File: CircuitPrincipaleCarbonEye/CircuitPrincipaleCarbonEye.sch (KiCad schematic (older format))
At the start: 28 parts, among them J1 Conn_01x01_Male, J2 4P4C, Q1 Q_PMOS_DGS, Q2 Q_NMOS_DGS, U1 OPA4227PA, U2 ADS1115, U3 GROOVE, U4 molex4-pin

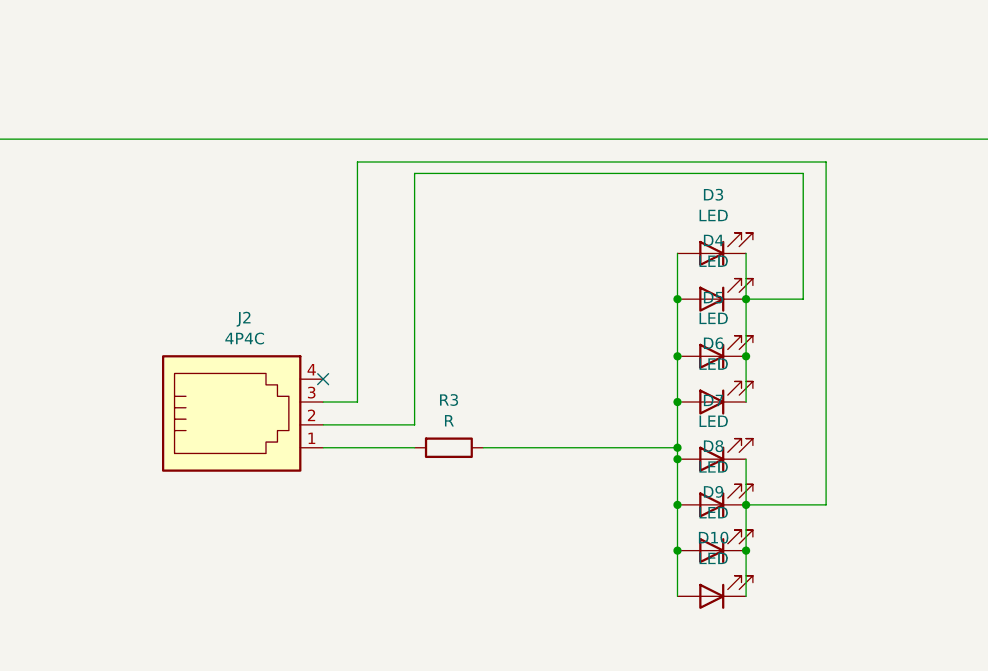
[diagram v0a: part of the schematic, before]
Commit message: CircuitLed V1.0
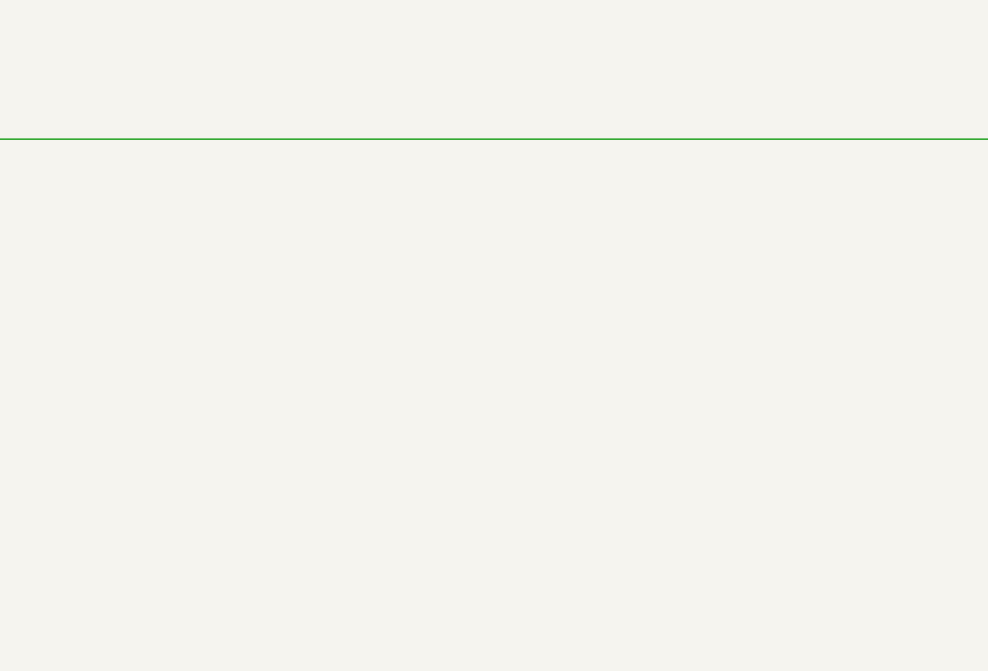
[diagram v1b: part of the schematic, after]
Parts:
- removed D10, D7, D8, D9: LED, symbol Device:LED
- removed D3, D4, D5, D6: LED, SamacSys_Parts:LEDM3528X185N, symbol Device:LED
- removed J2: 4P4C, symbol Connector:4P4C
- removed R3: R, symbol Device:R
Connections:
- no-connect marks 11 -> 10
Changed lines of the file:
@@
 Wire Wire Line
 	2150 5250 2450 5250
-$Comp
-L Connector:4P4C J2
-U 1 1 60EA57EE
-P 5950 4600
-F 0 "J2" H 6007 5067 50  0000 C CNN
-F 1 "4P4C" H 6007 4976 50  0000 C CNN
-F 2 "" V 5950 4650 50  0001 C CNN
-F 3 "~" V 5950 4650 50  0001 C CNN
-	1    5950 4600
-	1    0    0    -1
-$EndComp
-$Comp
-L Device:R R3
-U 1 1 60EA62A5
-P 6900 4700
-F 0 "R3" V 6693 4700 50  0000 C CNN
-F 1 "R" V 6784 4700 50  0000 C CNN
-F 2 "" V 6830 4700 50  0001 C CNN
-F 3 "~" H 6900 4700 50  0001 C CNN
-	1    6900 4700
-	0    1    1    0
-$EndComp
-$Comp
-L Device:LED D5
-U 1 1 60EA71C0
-P 8050 4300
-F 0 "D5" H 8043 4045 50  0000 C CNN
-F 1 "LED" H 8043 4136 50  0000 C CNN
-F 2 "SamacSys_Parts:LEDM3528X185N" H 8050 4300 50  0001 C CNN
-F 3 "~" H 8050 4300 50  0001 C CNN
-	1    8050 4300
-	-1   0    0    1
-$EndComp
-$Comp
-L Device:LED D4
-U 1 1 60EA7A9B
-P 8050 4050
-F 0 "D4" H 8043 3795 50  0000 C CNN
-F 1 "LED" H 8043 3886 50  0000 C CNN
-F 2 "SamacSys_Parts:LEDM3528X185N" H 8050 4050 50  0001 C CNN
-F 3 "~" H 8050 4050 50  0001 C CNN
-	1    8050 4050
-	-1   0    0    1
-$EndComp
-$Comp
-L Device:LED D3
-U 1 1 60EA7F32
-P 8050 3850
-F 0 "D3" H 8043 3595 50  0000 C CNN
-F 1 "LED" H 8043 3686 50  0000 C CNN
-F 2 "SamacSys_Parts:LEDM3528X185N" H 8050 3850 50  0001 C CNN
-F 3 "~" H 8050 3850 50  0001 C CNN
-	1    8050 3850
-	-1   0    0    1
-$EndComp
-$Comp
-L Device:LED D6
-U 1 1 60EA8289
-P 8050 4500
-F 0 "D6" H 8043 4245 50  0000 C CNN
-F 1 "LED" H 8043 4336 50  0000 C CNN
-F 2 "SamacSys_Parts:LEDM3528X185N" H 8050 4500 50  0001 C CNN
-F 3 "~" H 8050 4500 50  0001 C CNN
-	1    8050 4500
-	-1   0    0    1
-$EndComp
-Wire Wire Line
-	6350 4700 6750 4700
-Wire Wire Line
-	7900 3850 7900 4050
-Connection ~ 7900 4050
-Wire Wire Line
-	7900 4050 7900 4300
-Connection ~ 7900 4300
-Wire Wire Line
-	7900 4300 7900 4500
-Wire Wire Line
-	8200 3850 8200 4050
-Connection ~ 8200 4050
-Wire Wire Line
-	8200 4050 8200 4300
-Connection ~ 8200 4300
-Wire Wire Line
-	8200 4300 8200 4500
-$Comp
-L Device:LED D7
-U 1 1 60EB0F00
-P 8050 4750
-F 0 "D7" H 8043 4495 50  0000 C CNN
-F 1 "LED" H 8043 4586 50  0000 C CNN
-F 2 "" H 8050 4750 50  0001 C CNN
-F 3 "~" H 8050 4750 50  0001 C CNN
-	1    8050 4750
-	-1   0    0    1
-$EndComp
-$Comp
-L Device:LED D8
-U 1 1 60EB123F
-P 8050 4950
-F 0 "D8" H 8043 4695 50  0000 C CNN
-F 1 "LED" H 8043 4786 50  0000 C CNN
-F 2 "" H 8050 4950 50  0001 C CNN
-F 3 "~" H 8050 4950 50  0001 C CNN
-	1    8050 4950
-	-1   0    0    1
-$EndComp
-$Comp
-L Device:LED D9
-U 1 1 60EB143A
-P 8050 5150
-F 0 "D9" H 8043 4895 50  0000 C CNN
-F 1 "LED" H 8043 4986 50  0000 C CNN
-F 2 "" H 8050 5150 50  0001 C CNN
-F 3 "~" H 8050 5150 50  0001 C CNN
-	1    8050 5150
-	-1   0    0    1
-$EndComp
-$Comp
-L Device:LED D10
-U 1 1 60EB16ED
-P 8050 5350
-F 0 "D10" H 8043 5095 50  0000 C CNN
-F 1 "LED" H 8043 5186 50  0000 C CNN
-F 2 "" H 8050 5350 50  0001 C CNN
-F 3 "~" H 8050 5350 50  0001 C CNN
-	1    8050 5350
-	-1   0    0    1
-$EndComp
-Wire Wire Line
-	7900 4750 7900 4950
-Connection ~ 7900 4950
-Wire Wire Line
-	7900 4950 7900 5150
-Connection ~ 7900 5150
-Wire Wire Line
-	7900 5150 7900 5350
-Wire Wire Line
-	8200 4750 8200 4950
-Connection ~ 8200 4950
-Wire Wire Line
-	8200 4950 8200 5150
-Connection ~ 8200 5150
-Wire Wire Line
-	8200 5150 8200 5350
-Wire Wire Line
-	7050 4700 7900 4700
-Wire Wire Line
-	7900 4700 7900 4750
-Connection ~ 7900 4750
-Wire Wire Line
-	7900 4700 7900 4500
-Connection ~ 7900 4700
-Connection ~ 7900 4500
-Wire Wire Line
-	8200 4050 8450 4050
-Wire Wire Line
-	8450 4050 8450 3500
-Wire Wire Line
-	6750 3500 8450 3500
-Wire Wire Line
-	6350 4600 6750 4600
-Wire Wire Line
-	6750 3500 6750 4600
-Wire Wire Line
-	8200 4950 8550 4950
-Wire Wire Line
-	8550 4950 8550 3450
-Wire Wire Line
-	8550 3450 6500 3450
-Wire Wire Line
-	6500 3450 6500 4500
-Wire Wire Line
-	6500 4500 6350 4500
-NoConn ~ 6350 4400
 NoConn ~ 9100 1750
 NoConn ~ 9100 1850
